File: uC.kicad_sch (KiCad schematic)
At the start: 16 parts, among them J501 Conn_02x05_Counter_Clockwise, J502 Conn_02x08_Counter_Clockwise, J503 CLP-110-02-G-D, SW501 SW_Push, U501 BLUENRG-M2SA

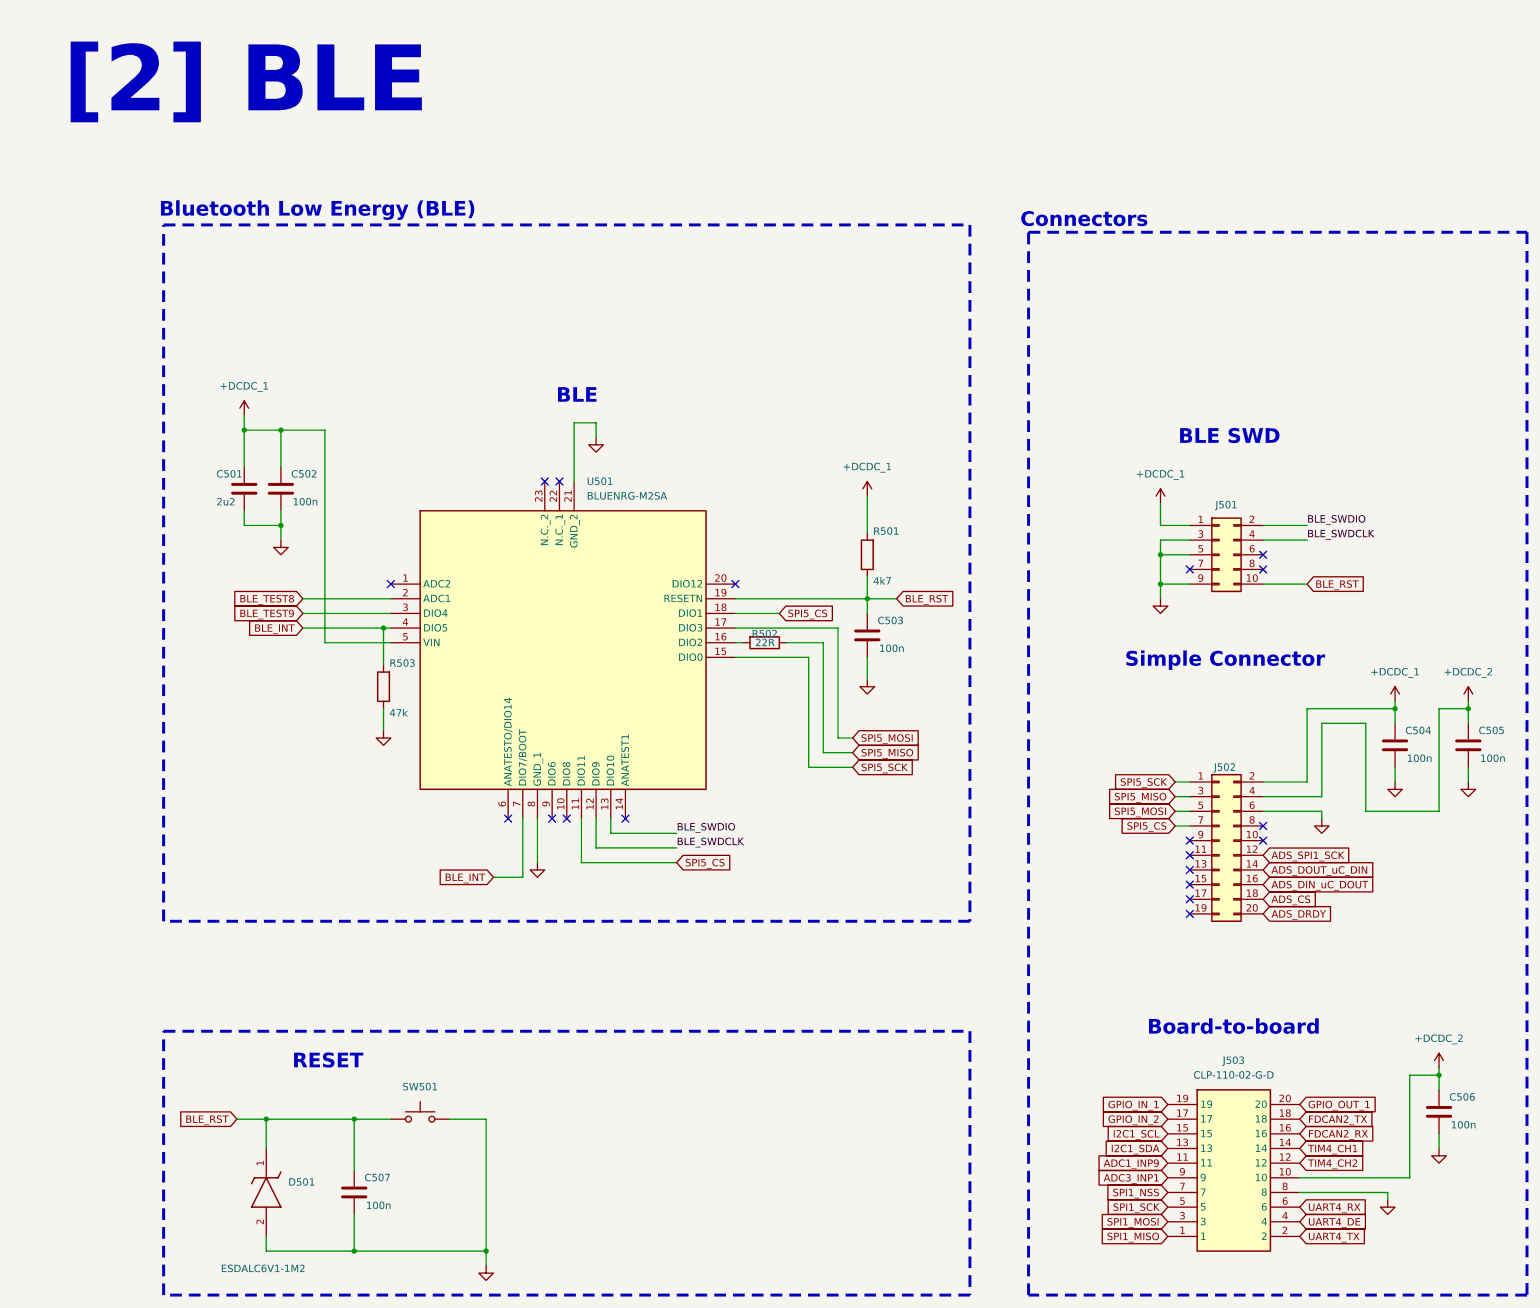
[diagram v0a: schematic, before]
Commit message: minor formatting updates
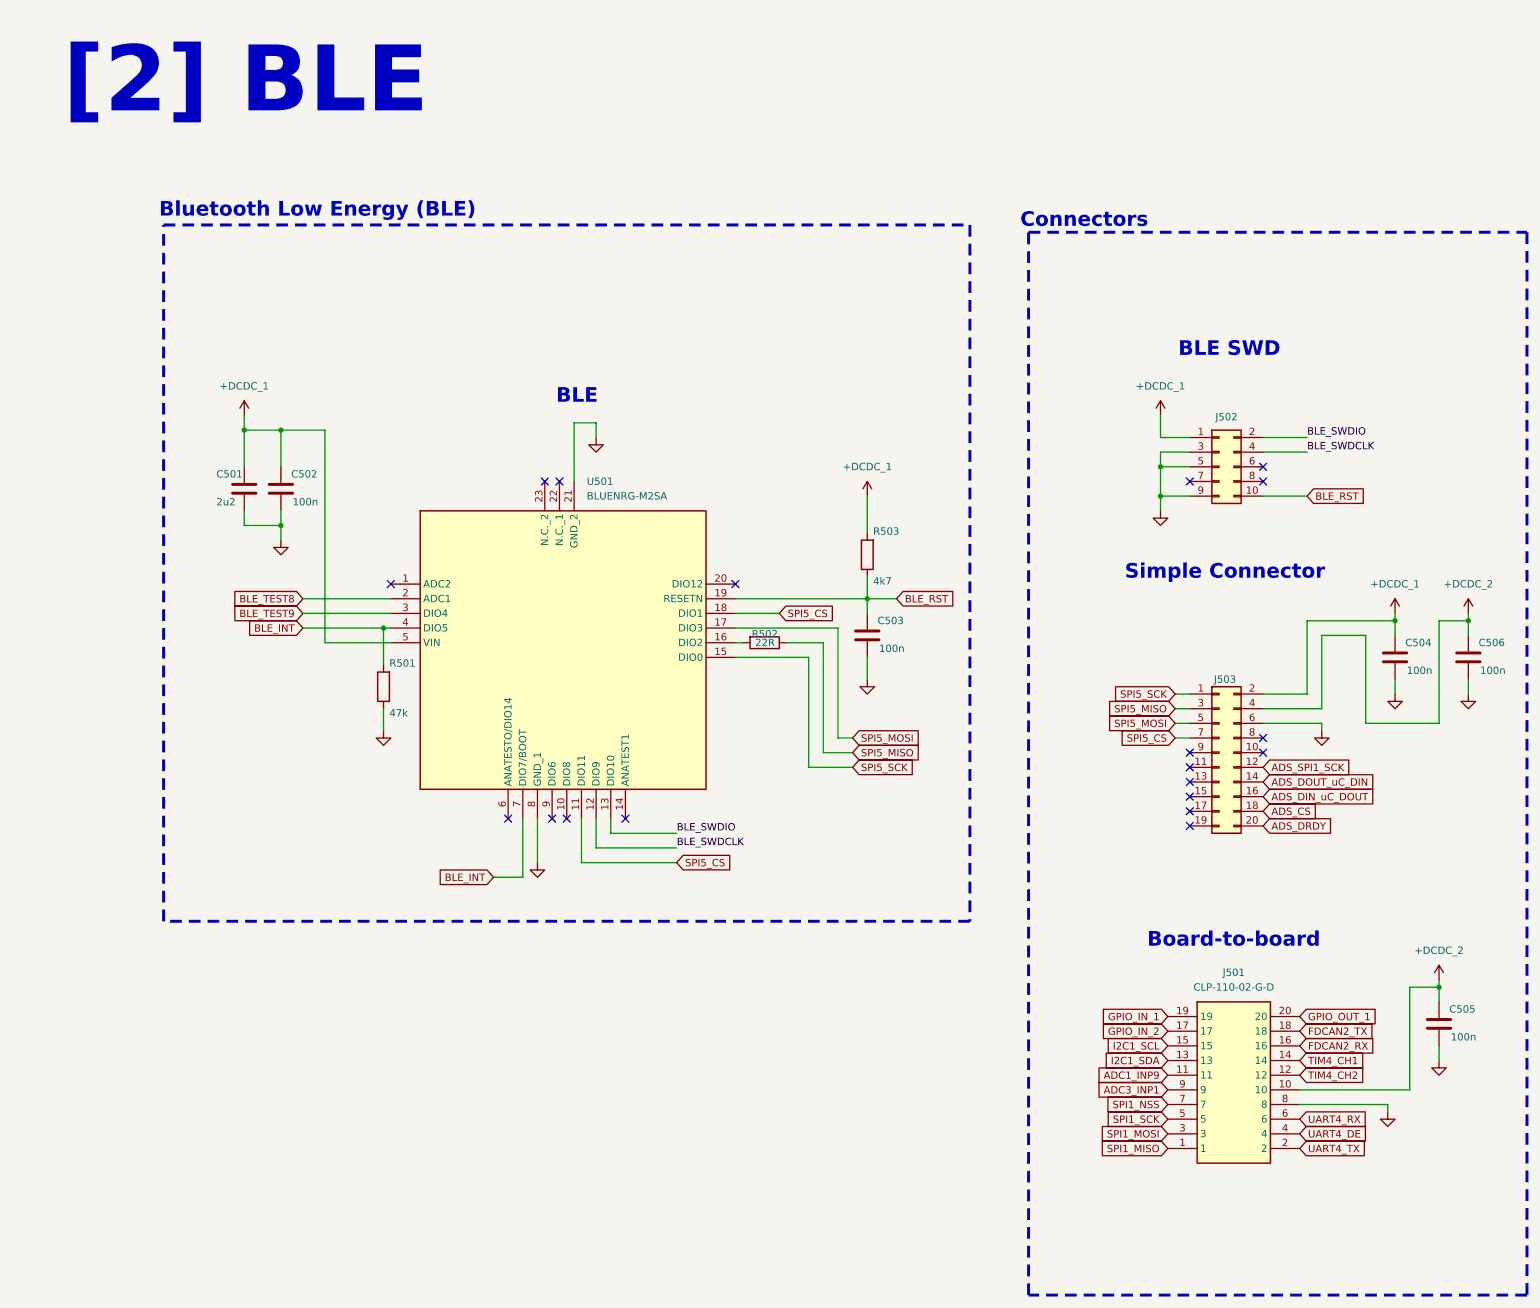
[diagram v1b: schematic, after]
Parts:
- removed C507: 100n, Capacitor_SMD:C_0402_1005Metric, symbol Device:C
- removed D501: ESDALC6V1-1M2, EMS:ESDALC6V11M2, symbol EMS:ESDALC6V1-1M2
- removed SW501: SW_Push, Button_Switch_SMD:SW_SPST_CK_RS282G05A3, symbol Switch:SW_Push
- renumbered C506 to C505, C505 to C506, J503 to J501, J501 to J502, J502 to J503, R503 to R501, R501 to R503
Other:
- note removed: "RESET"
- moved on the sheet: C504, C505, C506, J501, J502, J503
